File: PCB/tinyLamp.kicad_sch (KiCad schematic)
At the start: 26 parts, among them J11 Conn_01x02_Pin, J12 Conn_01x02_Pin, Q11 Q_NPN_BCE, Q12 Q_NPN_BCE, U11 WeMos_D1_mini

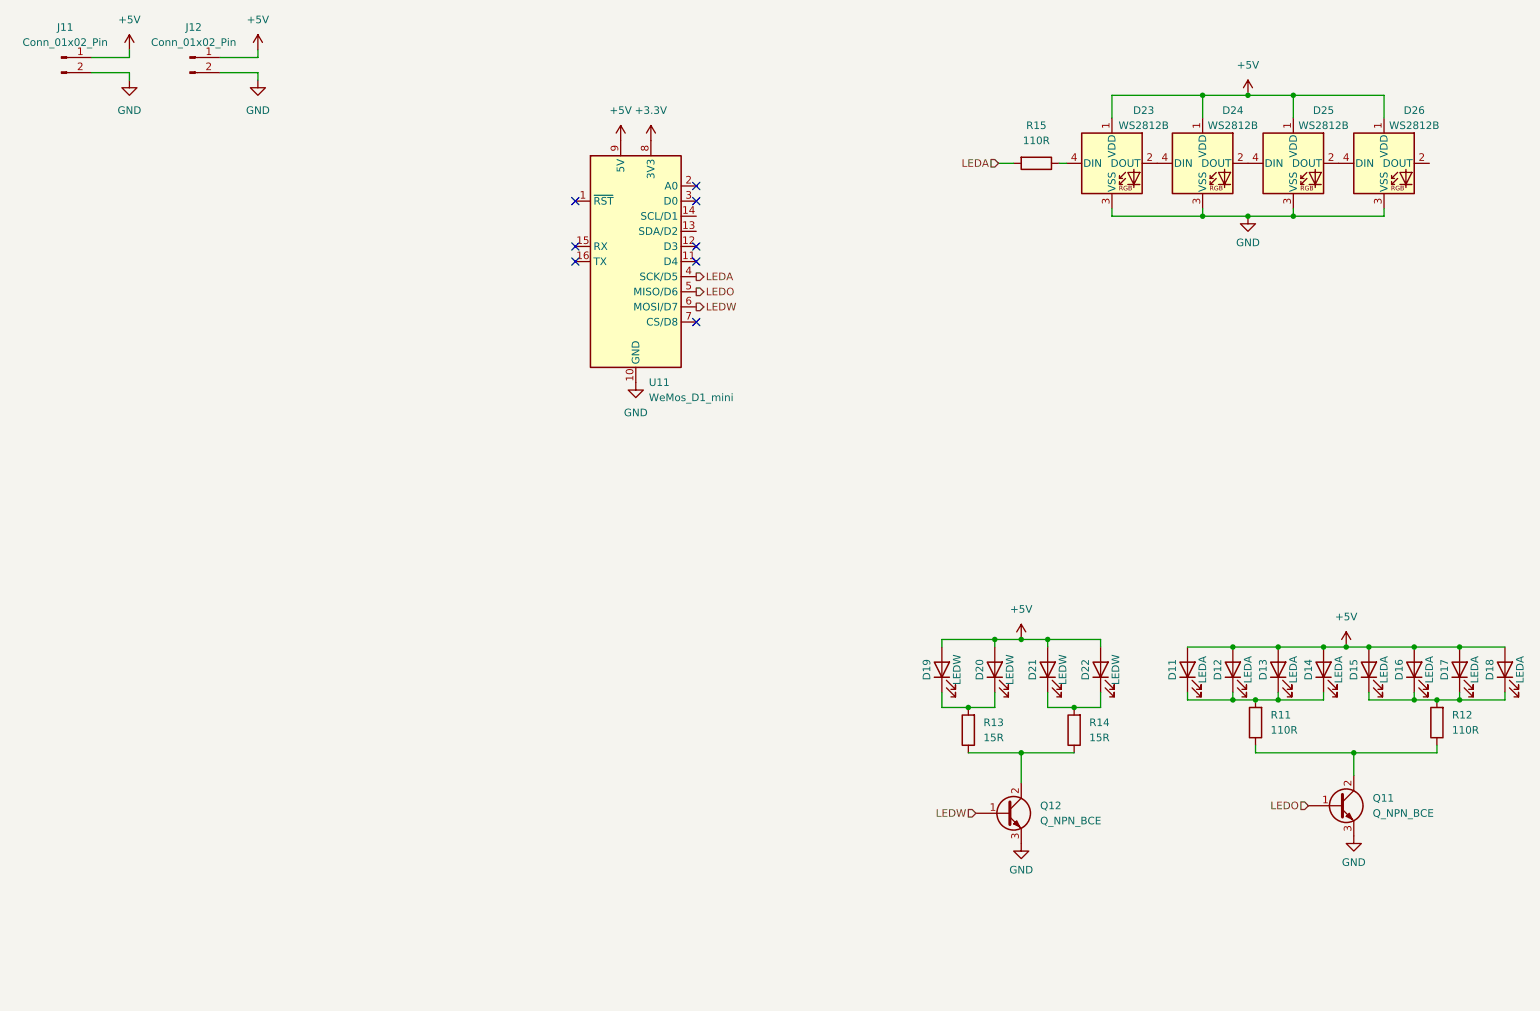
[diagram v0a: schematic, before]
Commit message: made some changes
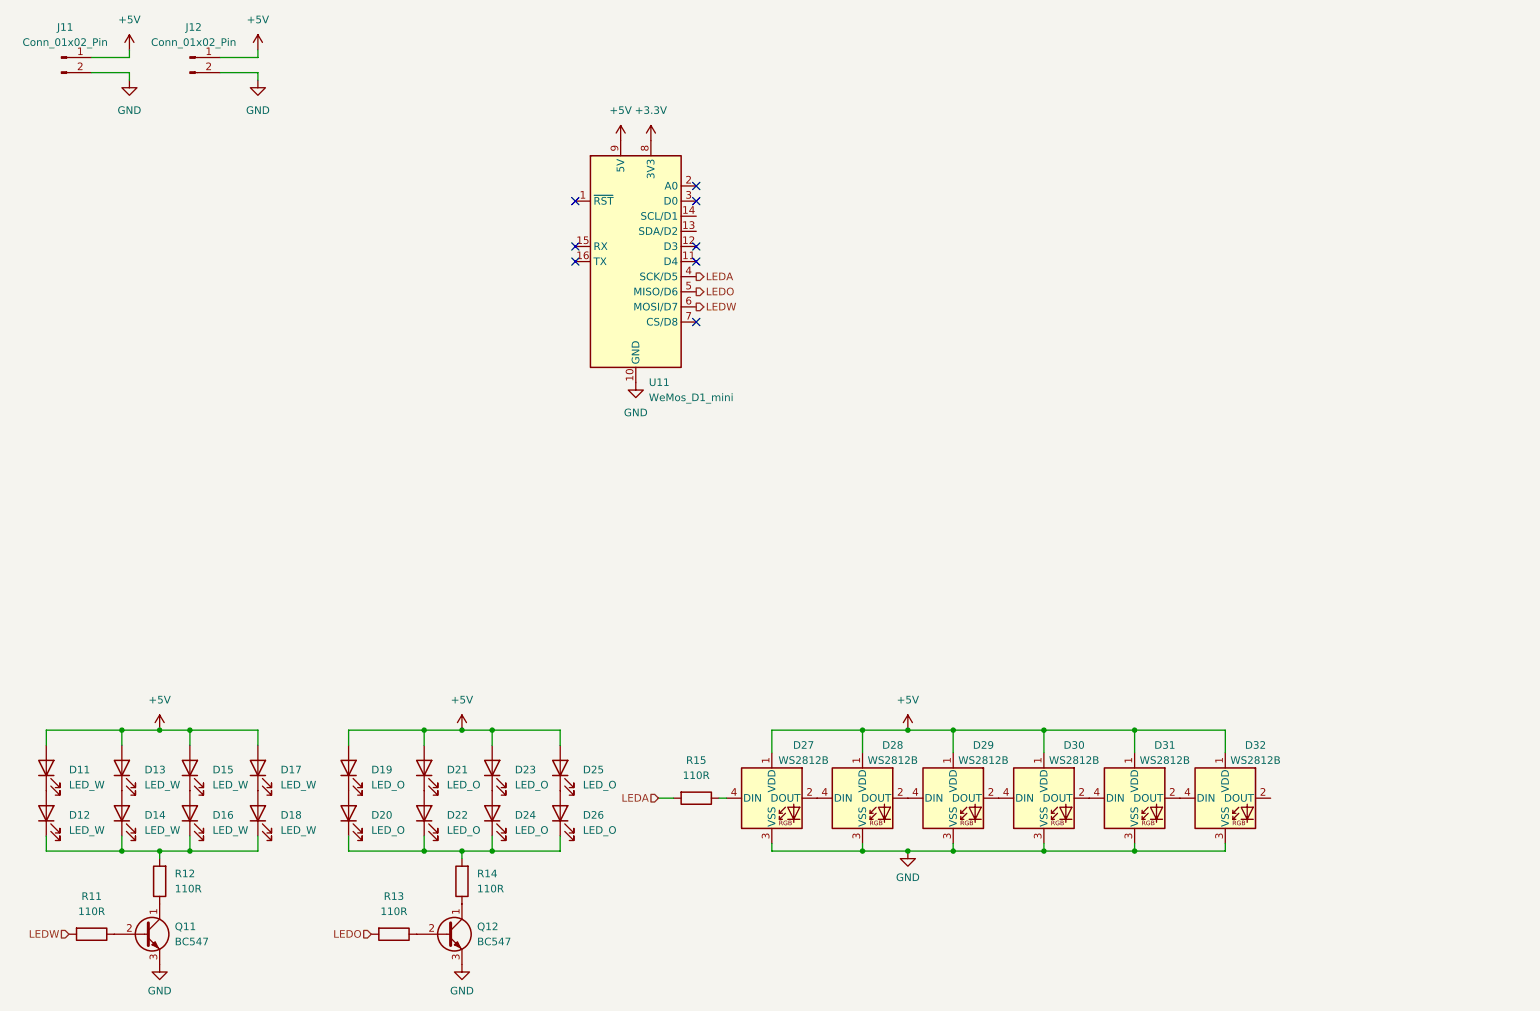
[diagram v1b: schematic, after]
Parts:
- removed Q11, Q12: Q_NPN_BCE, Package_TO_SOT_SMD:SOT-23, symbol Device:Q_NPN_BCE
- added D23, D24, D25, D26: LED_O, LED_THT:LED_D3.0mm_FlatTop, symbol Device:LED
- added D31, D32: WS2812B, LED_SMD:LED_WS2812B_PLCC4_5.0x5.0mm_P3.2mm, symbol LED:WS2812B
- added Q11, Q12: BC547, Package_TO_SOT_THT:TO-92L_HandSolder, symbol Transistor_BJT:BC547
- D11, D12, D13, D14, D15, D16, D17, D18: value LEDA -> LED_W; footprint LED_SMD:LED_0805_2012Metric_Pad1.15x1.40mm_HandSolder -> LED_THT:LED_D3.0mm_FlatTop; Price 0.017 -> (none)
- D19, D20, D21, D22: value LEDW -> LED_O; footprint LED_SMD:LED_PLCC-2 -> LED_THT:LED_D3.0mm_FlatTop; Price 0.010 -> (none)
- J11, J12: footprint (none) -> Connector_PinHeader_2.54mm:PinHeader_1x02_P2.54mm_Vertical
- R11, R12, R15: footprint Resistor_SMD:R_1206_3216Metric_Pad1.30x1.75mm_HandSolder -> Resistor_THT:R_Axial_DIN0207_L6.3mm_D2.5mm_P10.16mm_Horizontal
- R13, R14: value 15R -> 110R; footprint Resistor_SMD:R_1206_3216Metric_Pad1.30x1.75mm_HandSolder -> Resistor_THT:R_Axial_DIN0207_L6.3mm_D2.5mm_P10.16mm_Horizontal
- renumbered D23 to D27, D24 to D28, D25 to D29, D26 to D30
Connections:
- net +5V: now also D23.2 (A), D25.2 (A), D31.1 (VDD), D32.1 (VDD); no longer D12.2 (A), D14.2 (A), D16.2 (A), D18.2 (A), D20.2 (A), D22.2 (A)
- net GND: now also D31.3 (VSS), D32.3 (VSS), Q11.3 (E), Q12.3 (E)
- net LEDO: now also R13.2
- net LEDW: now also R11.2
- net at D16.1 (K), D18.1 (K), R12.2: now also D12.1 (K), D14.1 (K); no longer D15.1 (K), D17.1 (K)
- net at R12.1: now also Q11.1 (C); no longer R11.1
- net at R14.1: now also Q12.1 (C); no longer R13.1
- net at D22.1 (K), R14.2: now also D20.1 (K), D24.1 (K), D26.1 (K); no longer D21.1 (K)
- net at D30.2 (DOUT): now also D31.4 (DIN)
- new net: D31.2 (DOUT), D32.4 (DIN)
- new net: D25.1 (K), D26.2 (A)
- new net: D23.1 (K), D24.2 (A)
- new net: D13.1 (K), D14.2 (A)
- new net: Q11.2 (B), R11.1
- new net: Q12.2 (B), R13.1
- new net: D11.1 (K), D12.2 (A)
- new net: D19.1 (K), D20.2 (A)
- new net: D15.1 (K), D16.2 (A)
- new net: D17.1 (K), D18.2 (A)
- new net: D21.1 (K), D22.2 (A)
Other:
- moved on the sheet: D27, D28, D29, D30, R15
